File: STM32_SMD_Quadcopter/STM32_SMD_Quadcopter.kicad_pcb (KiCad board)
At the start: 2 copper layers, 36.5 x 25.4 mm, 61 parts, among them J1 PWR, J2 USB_B_Micro, J3 Micro_SD_Card_Det, J4 DEBUG, J5 DSMX, M1 Brushed_DC, M2 Brushed_DC, M3 Brushed_DC, M4 Brushed_DC, Q1 IRLML6244TR, Q2 IRLML6244TR, Q3 IRLML6244TR, Q4 IRLML6244TR, SW1 SW_Push, U1 LT1129-3.3_SOT223, U2 MPU-9250, U3 FT230XQ, U4 STM32F446RETx, Y1 8MHz ECS801830JGNTR

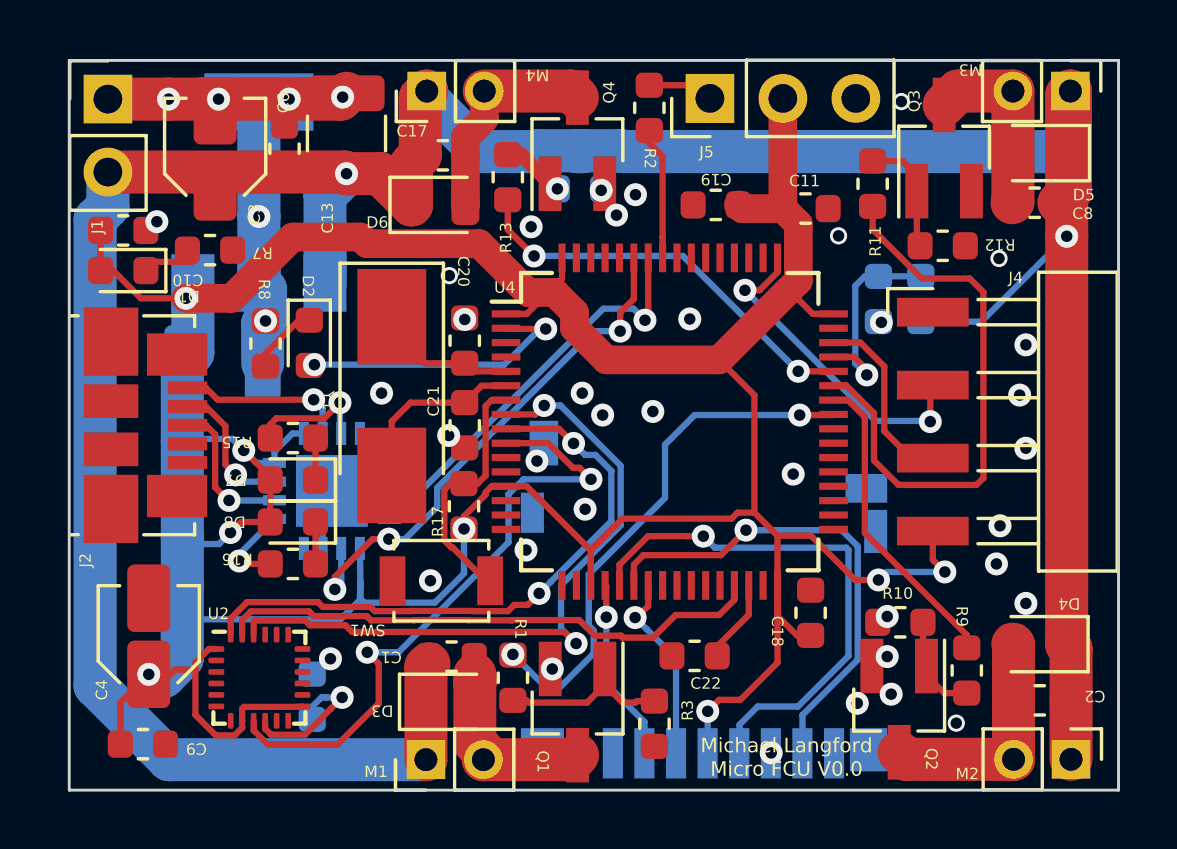
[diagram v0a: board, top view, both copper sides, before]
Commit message: All parts set in place
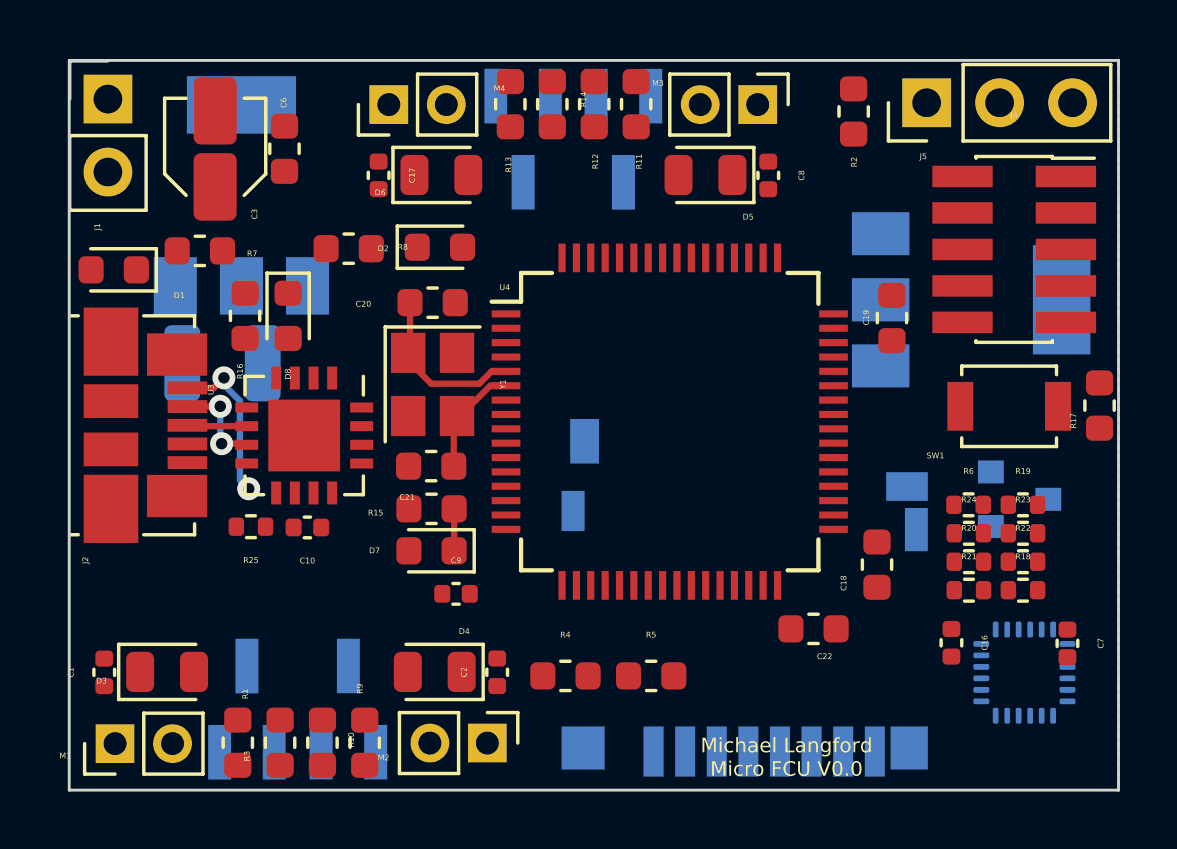
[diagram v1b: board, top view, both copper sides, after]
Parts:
- removed C11: 100nF, Capacitor_SMD:C_0603_1608Metric
- removed C13: 100uF, Capacitor_SMD:C_1210_3225Metric
- removed C4: 100uF, Capacitor_SMD:C_Elec_3x5.4
- added C16: 100nF, Capacitor_SMD:C_0402_1005Metric, F.Cu at (78.6, 48.2)
- added Q5: 2N7002, Package_TO_SOT_SMD:SOT-23, B.Cu at (81.0, 43.2)
- added R18: 1K, Resistor_SMD:R_0402_1005Metric, F.Cu at (81.1, 46.4)
- added R19: 1.2K, Resistor_SMD:R_0402_1005Metric, F.Cu at (81.1, 43.4)
- added R20: 1K, Resistor_SMD:R_0402_1005Metric, F.Cu at (79.2, 45.4)
- added R21: 10K, Resistor_SMD:R_0402_1005Metric, F.Cu at (79.2, 46.4)
- added R22: 1K, Resistor_SMD:R_0402_1005Metric, F.Cu at (81.1, 45.4)
- added R23: 1.2K, Resistor_SMD:R_0402_1005Metric, F.Cu at (81.1, 44.4)
- added R24: 1.2K, Resistor_SMD:R_0402_1005Metric, F.Cu at (79.2, 44.4)
- added R25: 22, Resistor_SMD:R_0402_1005Metric, F.Cu at (54.2, 44.2)
- added R6: 10K, Resistor_SMD:R_0402_1005Metric, F.Cu at (79.2, 43.4)
- added U5: ICM-20948, Sensor_Motion:InvenSense_QFN-24_3x3mm_P0.4mm, B.Cu at (81.2, 49.3)
- C1, C10, C17, C2, C8, C9: footprint Capacitor_SMD:C_0603_1608Metric -> Capacitor_SMD:C_0402_1005Metric
- C20, C21: value 22pF -> 12pF
- C7: footprint Capacitor_SMD:C_0603_1608Metric -> Capacitor_SMD:C_0402_1005Metric; moved to F.Cu
- J4: footprint STM32_SMD_Quadcopter:Harwin_M20-89004xx_1x04_P2.54mm_Horizontal_MODIFIEDSILKSCREEN -> Connector_PinSocket_1.27mm:PinSocket_2x05_P1.27mm_Vertical_SMD
- Q1, Q2, Q3, Q4: moved to B.Cu
- R14, U3: moved to F.Cu
- R15, R16: value 300 -> 2K
- R4: value 3K -> 30K; moved to F.Cu
- R5: value 10K -> 100K; moved to F.Cu
- R7, R8: value 470 -> 4.7k
- U1: value LT1129-3.3_SOT223 -> AMS1117-3.3
- U2: value MPU-9250 -> AMS1117-1.8; footprint Sensor_Motion:InvenSense_QFN-24_3x3mm_P0.4mm -> Package_TO_SOT_SMD:SOT-223-3_TabPin2; moved to B.Cu
- Y1: value 8MHz ECS801830JGNTR -> 16MHz X322516MLB4SI; footprint Crystal:Crystal_SMD_Abracon_ABM3-2Pin_5.0x3.2mm_HandSoldering -> Crystal:Crystal_SMD_3225-4Pin_3.2x2.5mm
- moved U2 28.1 mm to (79.3, 36.3)
- moved C7 26.4 mm to (82.7, 48.3), turned to 270 degrees
- moved R17 22.4 mm to (83.8, 40.0)
- moved R9 21.1 mm to (58.2, 51.7)
- moved D4 21.1 mm to (60.6, 49.3)
- moved SW1 20.7 mm to (80.6, 40.0)
- moved R10 20.5 mm to (56.7, 51.7), turned to 270 degrees
- moved M2 20.3 mm to (62.5, 51.7)
- moved Q2 19.2 mm to (57.6, 50.5), turned to 90 degrees
- moved C2 18.9 mm to (62.8, 49.3), turned to 90 degrees
- moved R4 18.0 mm to (65.2, 49.4), turned to 0 degrees
- moved R5 15.3 mm to (68.2, 49.4), turned to 0 degrees
- moved R12 13.1 mm to (66.2, 29.5), turned to 90 degrees
- moved R3 13.0 mm to (55.2, 51.7), turned to 270 degrees
- moved C10 12.2 mm to (56.2, 44.2)
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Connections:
- C10 pad 2: +3V3 -> Net-(C10-Pad2)
- C20 pad 1: GND -> Net-(C20-Pad1)
- C20 pad 2: Net-(C20-Pad2) -> GND
- C21 pad 1: GND -> Net-(C21-Pad1)
- C21 pad 2: Net-(C21-Pad2) -> GND
- J4 pad 1: GND -> +3V3
- J4 pad 2: SYS_JTCL-SWCLK -> SYS_JTMS-SWDIO
- J4 pad 3: SYS_JTMS-SWDIO -> GND
- J4 pad 4: +3V3 -> SYS_JTCL-SWCLK
- R17 pad 2: Net-(R17-Pad2) -> NRST
- SW1 pad 2: Net-(R17-Pad2) -> NRST
- U1 pad 1: +BATT -> GND
- U1 pad 2: GND -> +3V3
- U1 pad 3: +3V3 -> +BATT
- U2 pad 1: +3V3 -> GND
- U2 pad 2: (no net) -> +1V8
- U2 pad 3: (no net) -> +3V3
- U3 pad 8: +3V3 -> Net-(C10-Pad2)
- U3 pad 9: +3V3 -> Net-(C10-Pad2)
- U4 pad 5: Net-(C20-Pad2) -> Net-(C20-Pad1)
- U4 pad 6: Net-(C21-Pad2) -> Net-(C21-Pad1)
- U4 pad 7: Net-(R17-Pad2) -> NRST
- Y1 pad 1: Net-(C20-Pad2) -> Net-(C20-Pad1)
- Y1 pad 2: Net-(C21-Pad2) -> GND
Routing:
- net +3V3: track 137.8 -> 0.00 mm, vias 8 -> 0
- net +BATT: track 112.4 -> 0.00 mm, vias 2 -> 0
- net MPU9250_CS: track 24.3 -> 0.00 mm, vias 2 -> 0
- net SPI2_MISO: track 22.2 -> 0.00 mm, vias 2 -> 0
- net GND: track 22.2 -> 0.00 mm, vias 42 -> 0
- net SPI2_MOSI: track 21.5 -> 0.00 mm, vias 2 -> 0
- net MOTOR_C: track 19.7 -> 0.00 mm
- net SPI2_SCK: track 19.2 -> 0.00 mm
- net SPI1_SCK: track 18.8 -> 0.00 mm, vias 1 -> 0
- net USART1_RX: track 18.6 -> 0.00 mm, vias 3 -> 0
- net MOTOR_A: track 18.5 -> 0.00 mm, vias 2 -> 0
- net SPI1_MISO: track 17.2 -> 0.00 mm, vias 1 -> 0
- net MOTOR_D: track 14.4 -> 0.00 mm, vias 2 -> 0
- net USART1_TX: track 14.0 -> 0.00 mm, vias 1 -> 0
- net SYS_JTCL-SWCLK: track 11.5 -> 0.00 mm, vias 2 -> 0
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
